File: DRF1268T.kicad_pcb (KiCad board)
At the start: 2 copper layers, 26.2 x 34.8 mm, 10 parts, among them J1 SMA-J-P-X-RA-TH1, J2 Conn_01x08, J3 Conn_01x02_Male

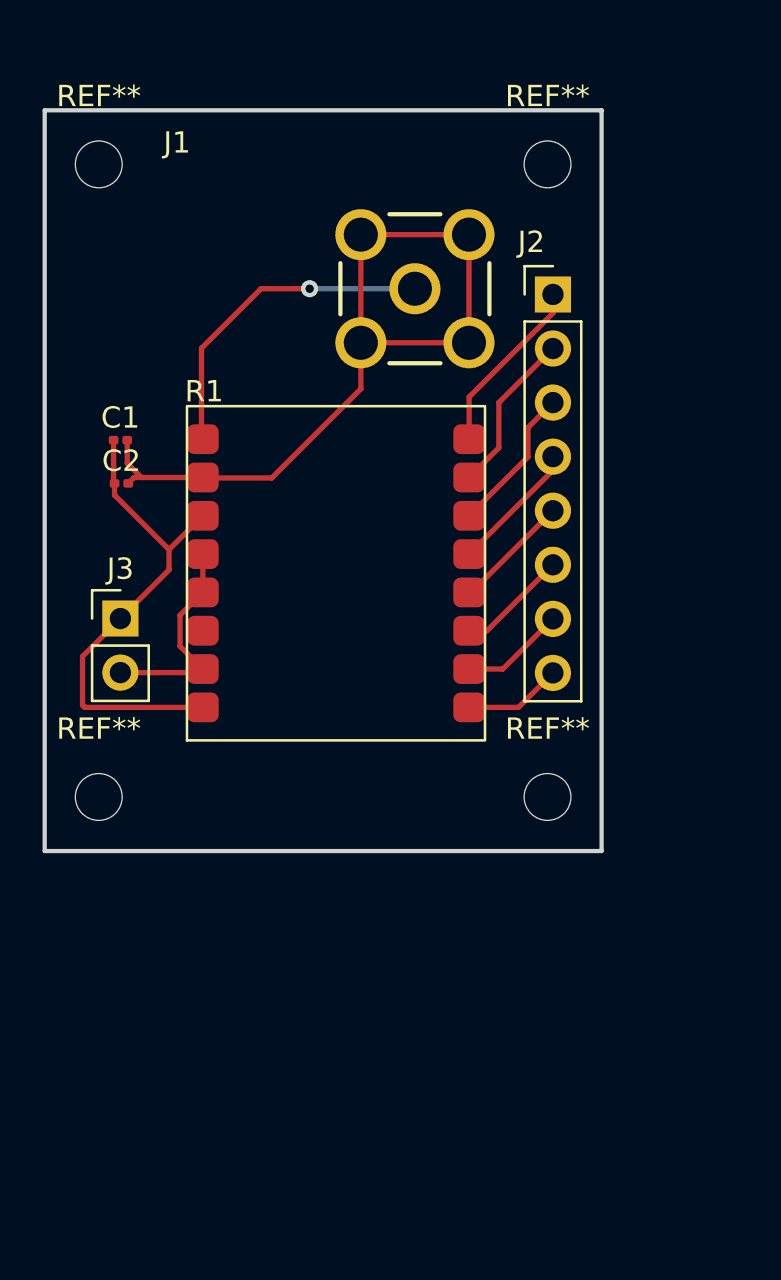
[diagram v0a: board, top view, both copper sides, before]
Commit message: Changes to pcb layout
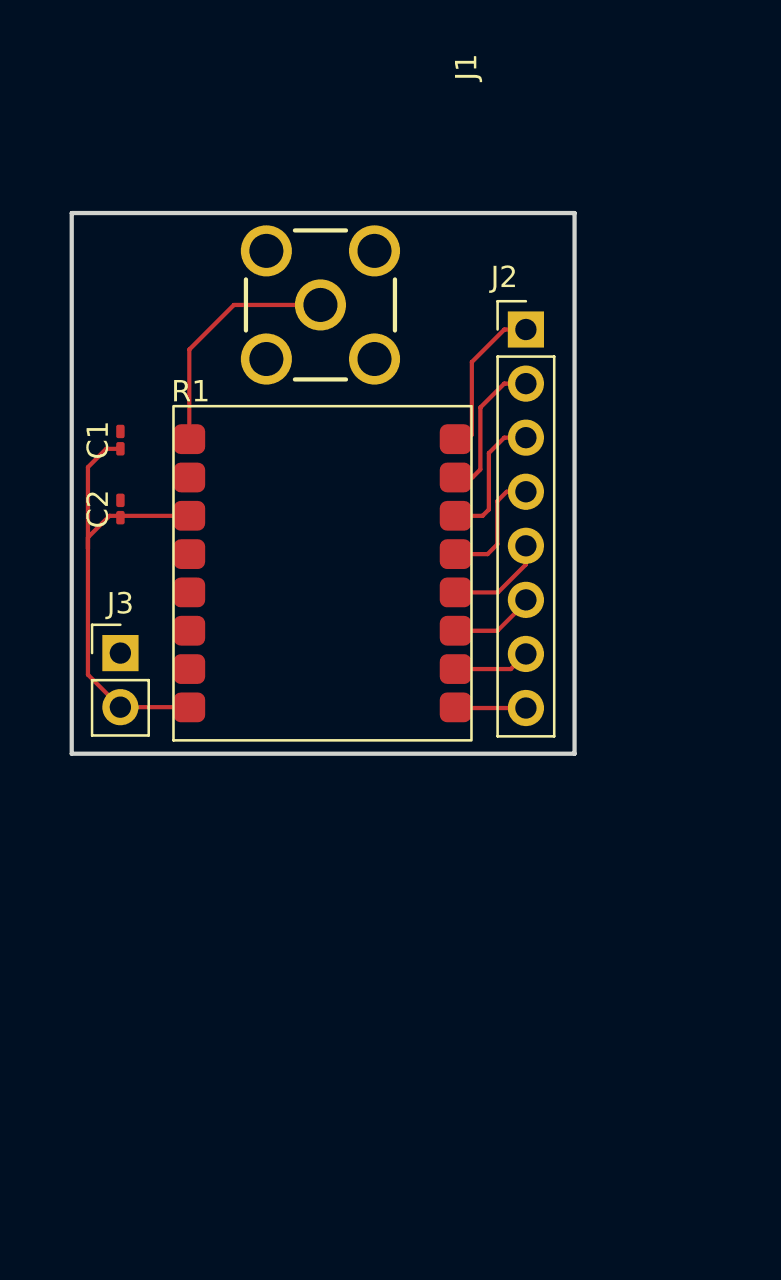
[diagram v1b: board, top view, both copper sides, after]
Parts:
- removed REF** (x4): MountingHole_2.2mm_M2, MountingHole:MountingHole_2.2mm_M2
- C1, C2: footprint Capacitor_SMD:C_0201_0603Metric -> Capacitor_SMD:C_0201_0603Metric_Pad0.64x0.40mm_HandSolder
- moved J1 4.50 mm to (151.6, 78.5), turned to -90 degrees
- moved J2 2.08 mm to (161.3, 79.6)
- moved J3 1.62 mm to (142.2, 94.8)
- moved C2 1.20 mm to (142.2, 88.1), turned to 90 degrees
- moved R1 0.63 mm to (144.7, 98.9)
- turned C1 to 90 degrees
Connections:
- J3 pad 1: +3.3V -> GND
- J3 pad 2: GND -> +3.3V
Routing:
- net GND: track 47.5 -> 0.00 mm
- net Net-(J1-Pad1): track 15.7 -> 11.2 mm, vias 1 -> 0
- net Net-(J2-Pad7): track 4.91 -> 3.60 mm
- net Net-(J2-Pad8): track 4.61 -> 3.31 mm
- net Net-(J2-Pad6): track 5.22 -> 3.97 mm
- net Net-(J2-Pad1): track 8.43 -> 7.44 mm
- net Net-(J2-Pad2): track 7.69 -> 6.83 mm
- net Net-(J2-Pad5): track 5.53 -> 4.72 mm
- net Net-(J2-Pad3): track 6.95 -> 6.38 mm
- net Net-(J2-Pad4): track 6.21 -> 5.71 mm
- added copper zone on B.Cu, net +3.3V
- added copper zone on F.Cu, net GND
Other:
- board size 26.2 x 34.8 mm -> 23.6 x 25.4 mm

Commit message: Changed
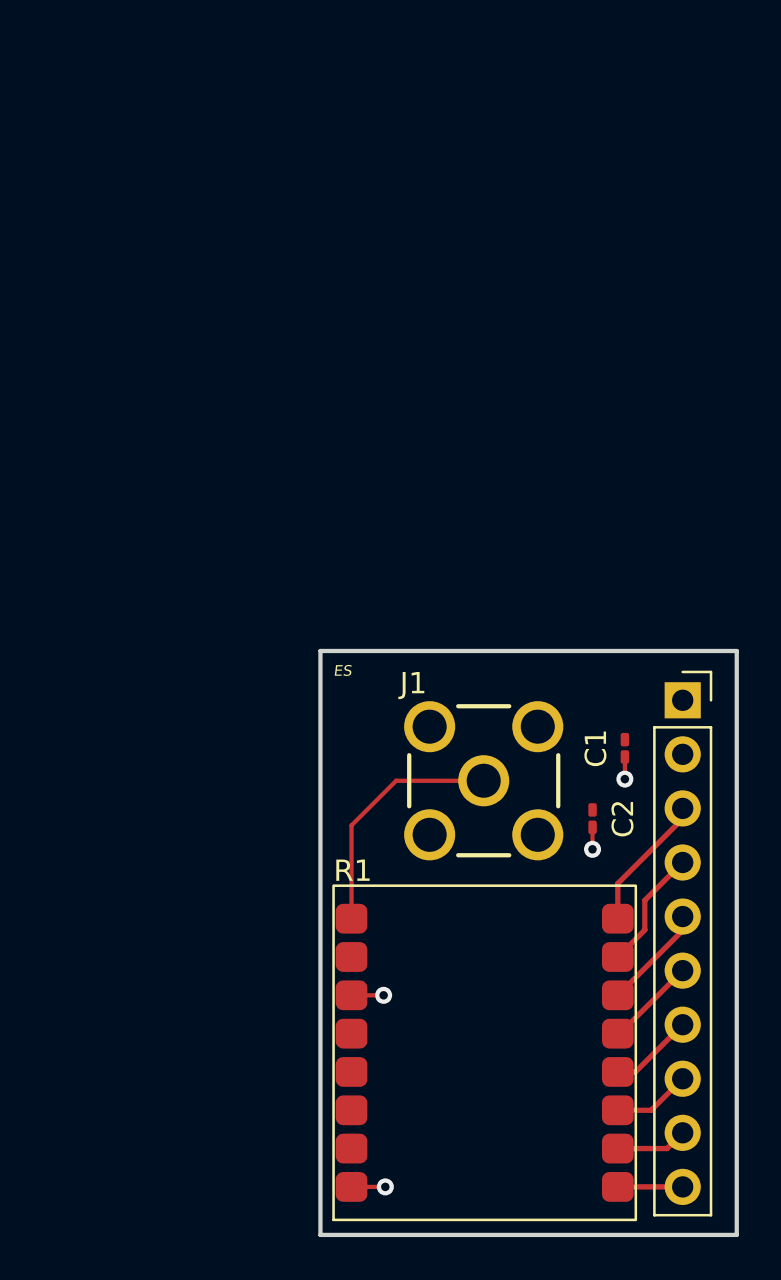
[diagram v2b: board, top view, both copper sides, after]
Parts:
- removed J3: Conn_01x02_Male, Connector_PinHeader_2.54mm:PinHeader_1x02_P2.54mm_Vertical
- C2: value C -> 10uF
- J2: value Conn_01x08 -> Conn_01x10_Male; footprint Connector_PinHeader_2.54mm:PinHeader_1x08_P2.54mm_Vertical -> Connector_PinSocket_2.54mm:PinSocket_1x10_P2.54mm_Vertical
- moved C1 27.8 mm to (165.9, 99.3)
- moved C2 26.5 mm to (164.4, 102.6)
- moved R1 23.8 mm to (152.4, 121.5)
- moved J1 23.6 mm to (159.3, 100.8)
- moved J2 18.9 mm to (168.7, 97.1)
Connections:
- J2 pad 1: Net-(J2-Pad1) -> +3.3V
- J2 pad 2: Net-(J2-Pad2) -> GND
- J2 pad 3: Net-(J2-Pad3) -> Net-(R1-Pad16)
- J2 pad 4: Net-(J2-Pad4) -> Net-(R1-Pad15)
- J2 pad 5: Net-(J2-Pad5) -> Net-(R1-Pad14)
- J2 pad 6: Net-(J2-Pad6) -> Net-(R1-Pad13)
- J2 pad 7: Net-(J2-Pad7) -> Net-(R1-Pad12)
- J2 pad 8: Net-(J2-Pad8) -> Net-(R1-Pad11)
- R1 pad 10: Net-(J2-Pad7) -> Net-(R1-Pad10)
- R1 pad 11: Net-(J2-Pad6) -> Net-(R1-Pad11)
- R1 pad 12: Net-(J2-Pad5) -> Net-(R1-Pad12)
- R1 pad 13: Net-(J2-Pad4) -> Net-(R1-Pad13)
- R1 pad 14: Net-(J2-Pad3) -> Net-(R1-Pad14)
- R1 pad 15: Net-(J2-Pad2) -> Net-(R1-Pad15)
- R1 pad 16: Net-(J2-Pad1) -> Net-(R1-Pad16)
- R1 pad 9: Net-(J2-Pad8) -> Net-(R1-Pad9)
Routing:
- net +3.3V: track 22.7 -> 5.17 mm, vias 0 -> 4
- net Net-(J2-Pad1): track 7.44 -> 0.00 mm
- net Net-(J2-Pad2): track 6.83 -> 0.00 mm
- net Net-(R1-Pad16): track 0.00 -> 6.44 mm
- net Net-(J2-Pad3): track 6.38 -> 0.00 mm
- net Net-(J2-Pad4): track 5.71 -> 0.00 mm
- net Net-(R1-Pad15): track 0.00 -> 5.70 mm
- net Net-(R1-Pad14): track 0.00 -> 4.96 mm
- net Net-(J2-Pad5): track 4.72 -> 0.00 mm
- net Net-(R1-Pad13): track 0.00 -> 4.27 mm
- net Net-(J2-Pad6): track 3.97 -> 0.00 mm
- net Net-(R1-Pad12): track 0.00 -> 3.97 mm
- net Net-(R1-Pad11): track 0.00 -> 3.66 mm
- net Net-(J2-Pad7): track 3.60 -> 0.00 mm
- net Net-(R1-Pad10): track 0.00 -> 3.35 mm
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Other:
- board size 23.6 x 25.4 mm -> 19.6 x 27.4 mm
- board text added: "ES"

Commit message: edits
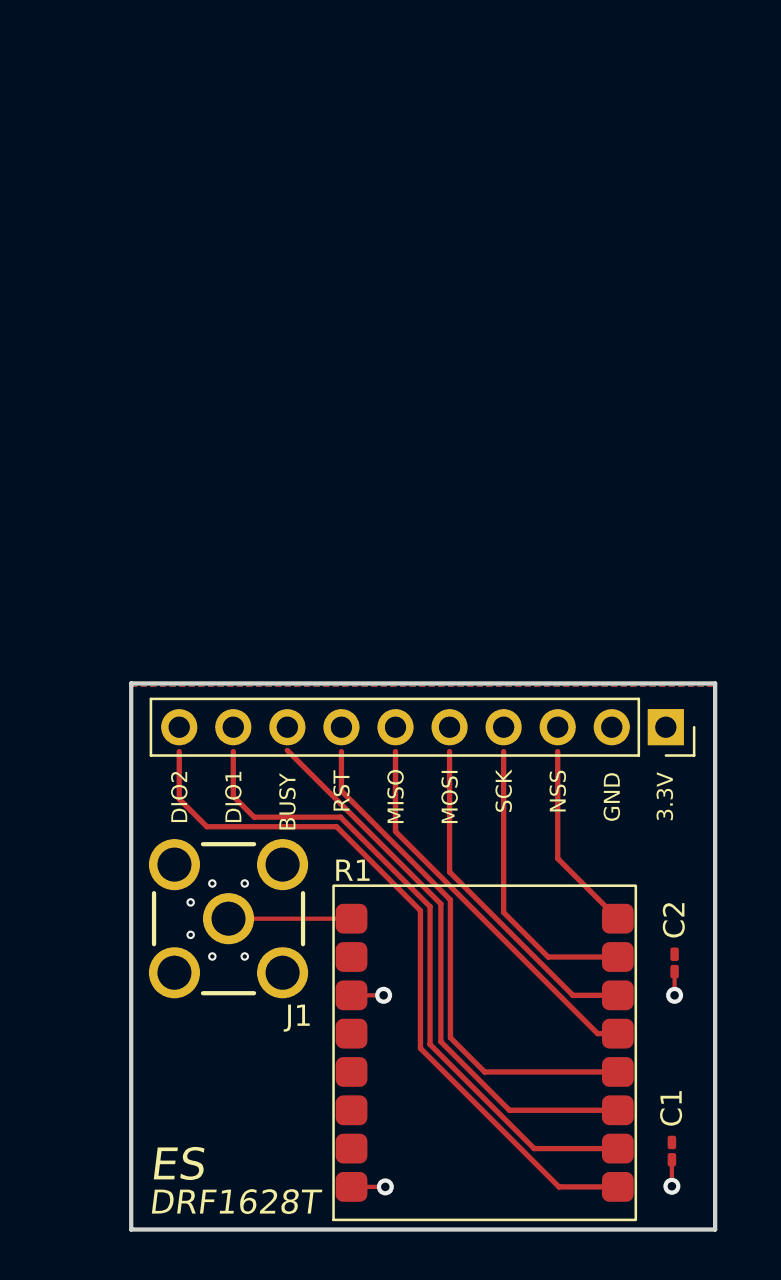
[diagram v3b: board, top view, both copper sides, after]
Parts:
- moved C1 19.1 mm to (168.1, 118.2)
- moved J1 13.6 mm to (147.3, 107.3), turned to 90 degrees
- moved C2 7.80 mm to (168.3, 109.4)
- moved J2 1.49 mm to (167.9, 98.3), turned to -90 degrees
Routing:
- net Net-(R1-Pad9): track 3.05 -> 34.2 mm
- net Net-(R1-Pad10): track 3.35 -> 30.8 mm
- net Net-(R1-Pad11): track 3.66 -> 26.3 mm
- net Net-(R1-Pad12): track 3.97 -> 24.1 mm
- net Net-(R1-Pad13): track 4.27 -> 18.1 mm
- net Net-(R1-Pad14): track 4.96 -> 16.0 mm
- net Net-(R1-Pad15): track 5.70 -> 13.8 mm
- net Net-(J1-Pad1): track 11.2 -> 5.78 mm
- net Net-(R1-Pad16): track 6.44 -> 9.02 mm
- net GND: vias 0 -> 6
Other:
- board size 19.6 x 27.4 mm -> 27.4 x 25.7 mm
- board text added: "3.3V"
- board text added: "BUSY"
- board text added: "DIO1"
- board text added: "DIO2"
- board text added: "DRF1628T"
- board text added: "GND"
- board text added: "MISO"
- board text added: "MOSI"
- board text added: "NSS"
- board text added: "RST"
- board text added: "SCK"
